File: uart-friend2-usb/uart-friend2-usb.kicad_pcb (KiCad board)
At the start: 4 copper layers, 56.5 x 15.5 mm, 58 parts, among them J1 USB_C_Receptacle_USB2.0, J2 Conn_02x03_Odd_Even, P1 USB_A_Plug_PCB, P2 USB_C_Plug_USB2.0_16P, P3 USB_C_Plug_USB2.0_16P, P4 USB_C_Plug_USB3.0_9P, SW1 BOOT, SW2 RST, U1 RP2040, U2 W25Q128JVPIQ, U3 WE-TVS-82400102, U4 AP7366-33W5-7, U5 WE-TVS-82400102, Y1 12MHz

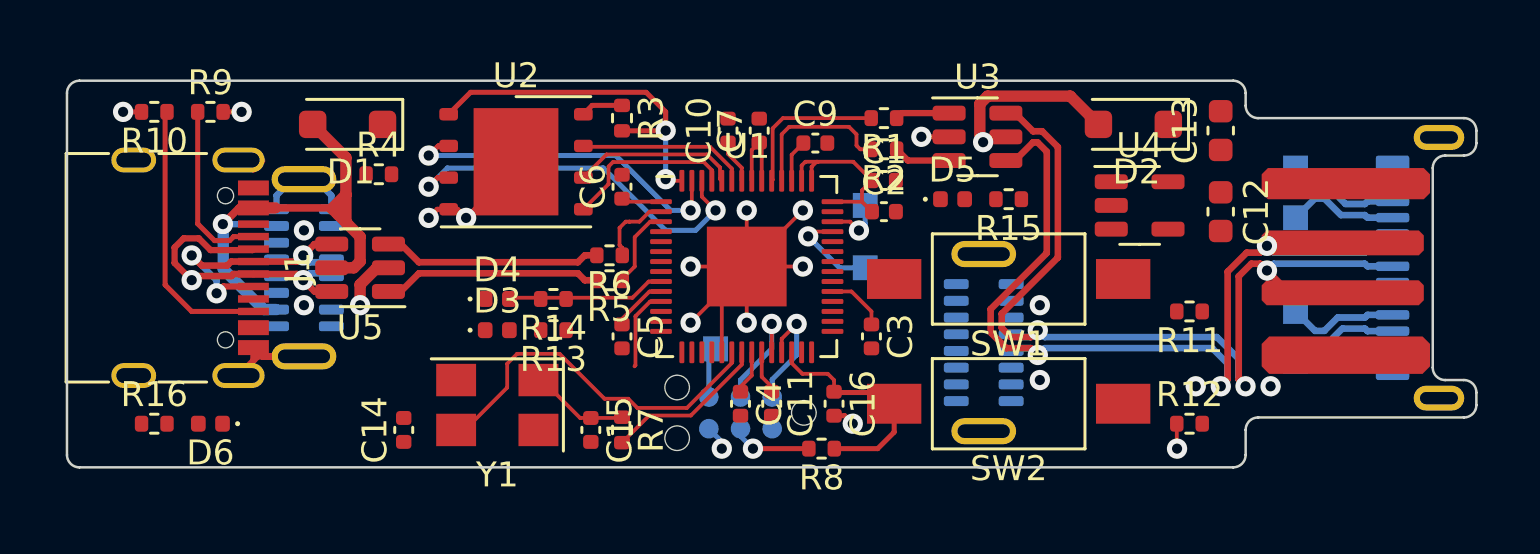
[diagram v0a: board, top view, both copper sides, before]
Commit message: uart-friend2-usb R1 layout schematic metadata production files
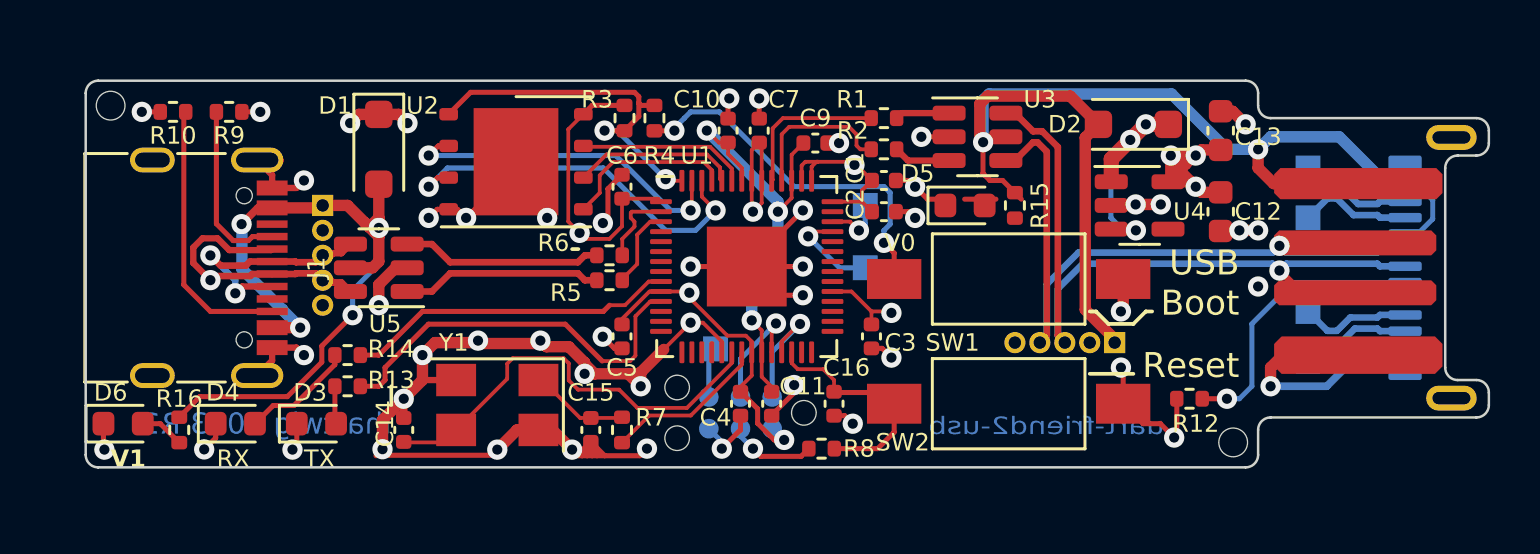
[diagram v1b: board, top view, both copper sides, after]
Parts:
- removed R11: 5.1k, Resistor_SMD:R_0402_1005Metric
- added REF**: MountingHole_1.152mm_JLCPCB_Tooling, uart-friend2-usb-special:MountingHole_1.152mm_JLCPCB_Tooling, F.Cu at (171.0, 114.5)
- added REF**: MountingHole_1.152mm_JLCPCB_Tooling, uart-friend2-usb-special:MountingHole_1.152mm_JLCPCB_Tooling, F.Cu at (126.0, 101.0)
- C14, C15: value 16pF -> 15pF
- D3, D4: value Orange -> Yellow; footprint LED_SMD:LED_0402_1005Metric -> LED_SMD:LED_0603_1608Metric
- D5, D6: footprint LED_SMD:LED_0402_1005Metric -> LED_SMD:LED_0603_1608Metric
- P2, P3: footprint uart-friend2-usb-special:USB_C_Plug_YIYUAN_YTC-TC16S-128_16P_Vertical -> Connector_PinHeader_1.00mm:PinHeader_1x05_P1.00mm_Vertical
- R7: value 7.2k -> 6.8k
- moved D4 11.6 mm to (131.0, 113.8)
- moved R4 11.3 mm to (147.8, 101.5), turned to 90 degrees
- moved R13 8.55 mm to (135.5, 112.2)
- moved R14 8.55 mm to (135.5, 111.0)
- moved D3 8.16 mm to (134.2, 113.8)
- moved P2 5.25 mm to (166.2, 110.5)
- moved D6 3.50 mm to (126.5, 113.8), turned to 0 degrees
- moved P3 2.61 mm to (134.5, 105.0), turned to 180 degrees
- moved D1 1.60 mm to (136.8, 102.8), turned to -90 degrees
- moved R16 1.03 mm to (128.8, 114.0), turned to -90 degrees
- moved R12 1.00 mm to (169.2, 112.8)
- moved J1 0.75 mm to (128.8, 107.5)
- moved R10 0.75 mm to (128.5, 101.2)
- moved R9 0.75 mm to (130.8, 101.2)
- moved U5 0.75 mm to (136.8, 107.5)
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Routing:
- net GND: track 53.3 -> 115.1 mm, vias 21 -> 48
- net /VBUS0: track 7.95 -> 49.8 mm, vias 1 -> 2
- net +3V3: track 20.2 -> 50.1 mm, vias 0 -> 9
- net /U1_BOOT: track 0.00 -> 15.1 mm, vias 0 -> 2
- net VDD: track 5.02 -> 18.2 mm, vias 0 -> 3
- net /LED_GPIO8: track 3.29 -> 15.9 mm
- net VBUS: track 0.00 -> 12.0 mm, vias 0 -> 5
- net /P4_CC: track 0.00 -> 11.5 mm, vias 0 -> 1
- net /VBUS1: track 21.5 -> 30.5 mm, vias 1 -> 4
- net /USB0_D_N: track 34.7 -> 27.5 mm, vias 3 -> 1
- net /USB0_D_P: track 38.1 -> 30.9 mm, vias 3 -> 1
- net /LED_GPIO7: track 6.32 -> 13.3 mm
- net Net-(D4-A): track 0.00 -> 4.56 mm
- net /U1_XIN: track 14.9 -> 17.3 mm
- net Net-(D6-A): track 0.00 -> 1.78 mm
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- added copper zone on In2.Cu, net +3V3
- added copper zone on In2.Cu, net VBUS
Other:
- board size 56.5 x 15.5 mm -> 56.2 x 15.5 mm
- board text added: "CC"
- board text added: "RX"
- board text added: "RX1N"
- board text added: "Reset"
- board text added: "SWD Dbg"
- board text added: "TX"
- board text added: "TX1P"
- board text added: "USB Boot"
- board text added: "V0"
- board text added: "V1"
- board text added: "VG+-G"
- board text added: "ihartwig 2023 R1"
- board text added: "uart-friend2-usb"
